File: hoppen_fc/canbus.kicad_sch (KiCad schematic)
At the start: 8 parts, among them U13 TJA1051TK-3, U14 TJA1051TK-3

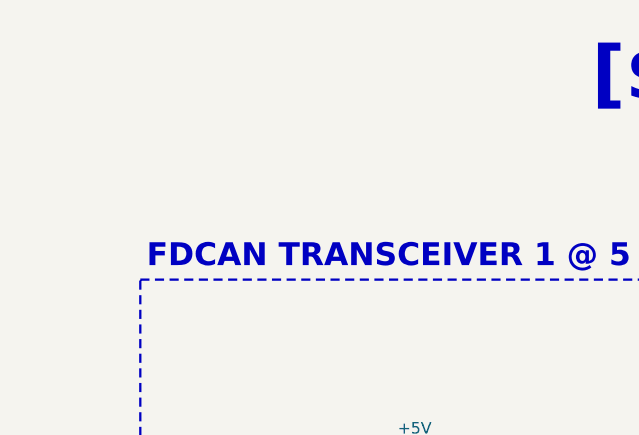
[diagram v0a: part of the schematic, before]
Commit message: comments
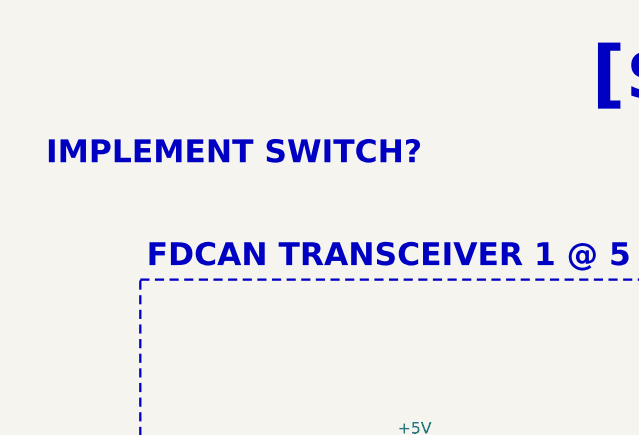
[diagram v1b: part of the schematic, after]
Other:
- note added: "IMPLEMENT SWITCH?"
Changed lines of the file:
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@@
+		)
+	)
+	(text "IMPLEMENT SWITCH?"
+		(exclude_from_sim no)
+		(at 66.294 38.1 0)
+		(effects
+			(font
+				(face "KiCad Font")
+				(size 2.54 2.54)
+				(thickness 0.508)
+				(bold yes)
+				(color 255 0 0 1)
+			)
 		)
 	)

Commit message: bump
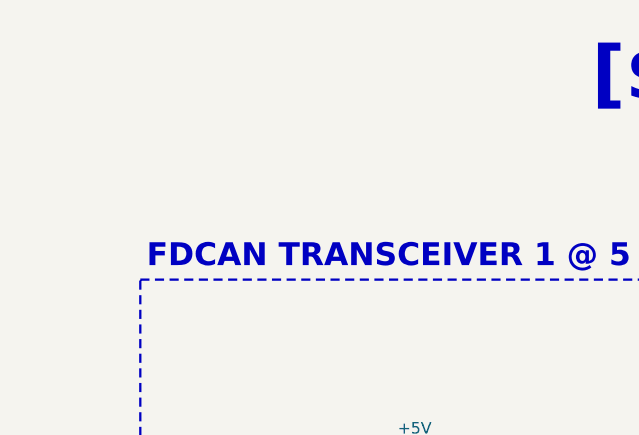
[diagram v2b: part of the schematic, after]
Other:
- note removed: "IMPLEMENT SWITCH?"
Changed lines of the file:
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@@
-		)
-	)
-	(text "IMPLEMENT SWITCH?"
-		(exclude_from_sim no)
-		(at 66.294 38.1 0)
-		(effects
-			(font
-				(face "KiCad Font")
-				(size 2.54 2.54)
-				(thickness 0.508)
-				(bold yes)
-				(color 255 0 0 1)
-			)
 		)
 	)
